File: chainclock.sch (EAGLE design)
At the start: 15 parts

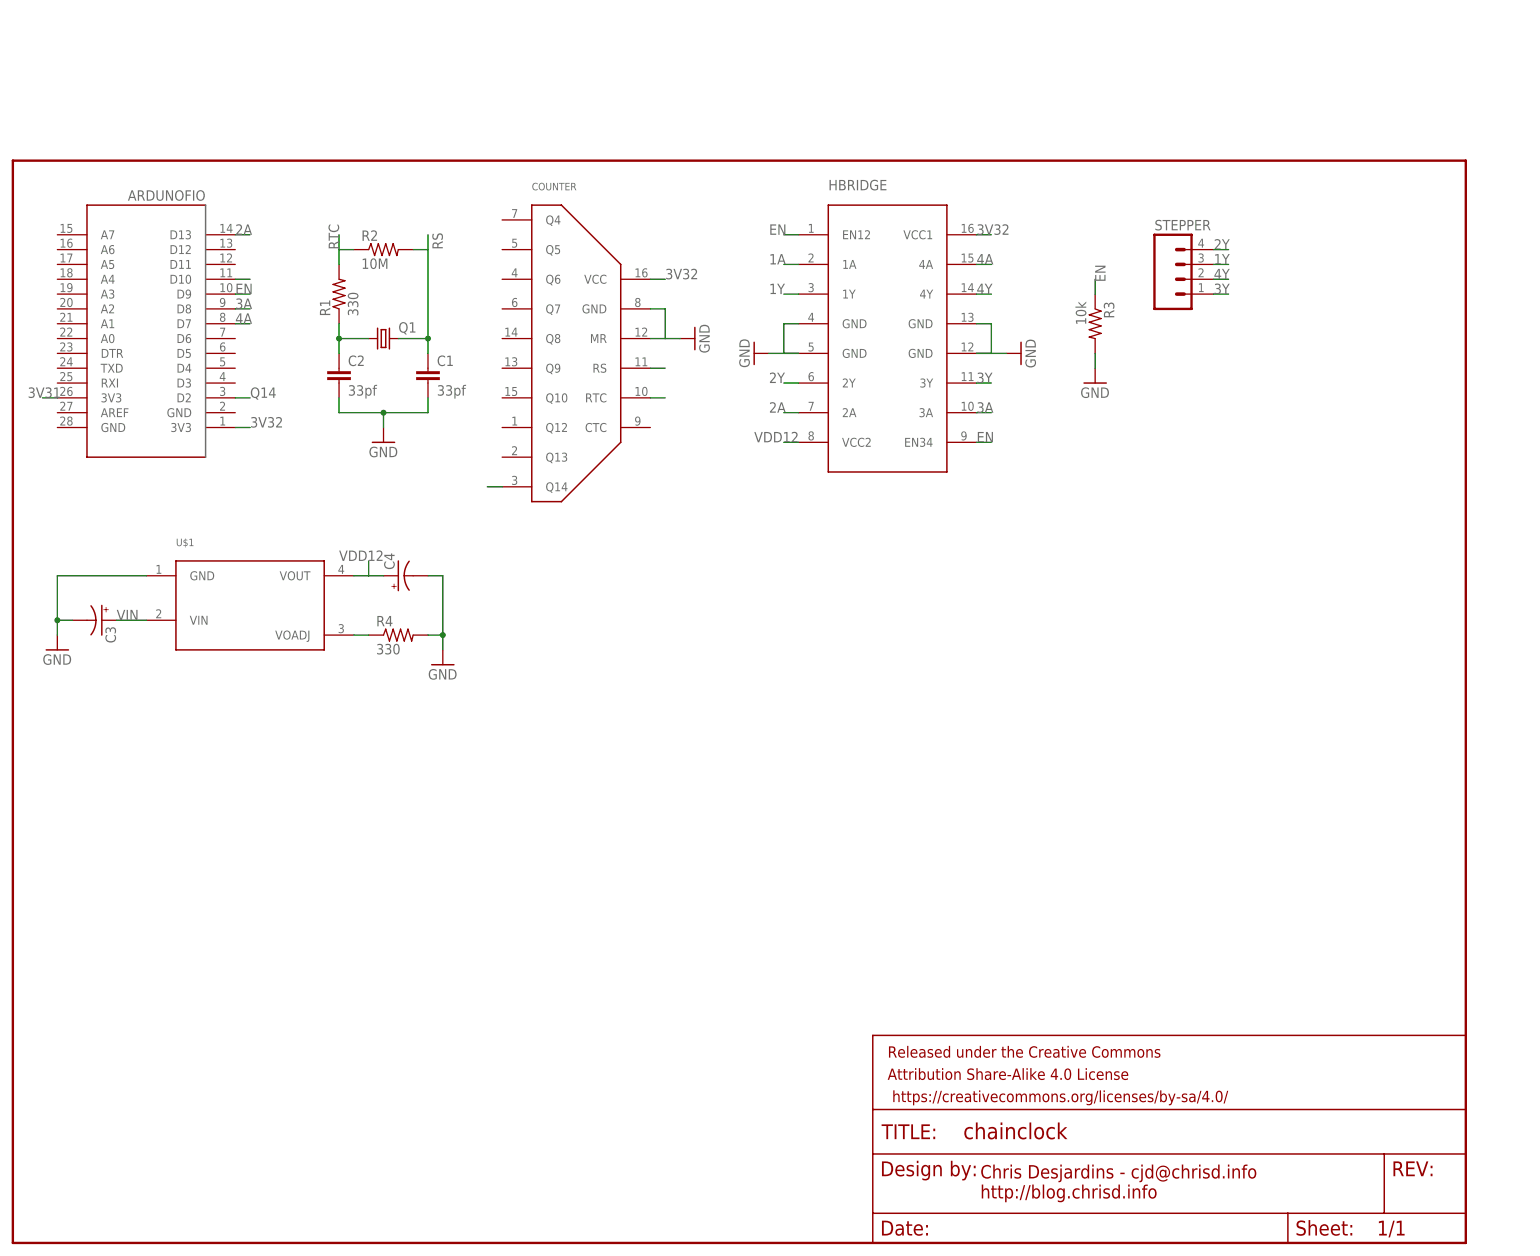
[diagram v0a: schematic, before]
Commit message: Move some stuff around
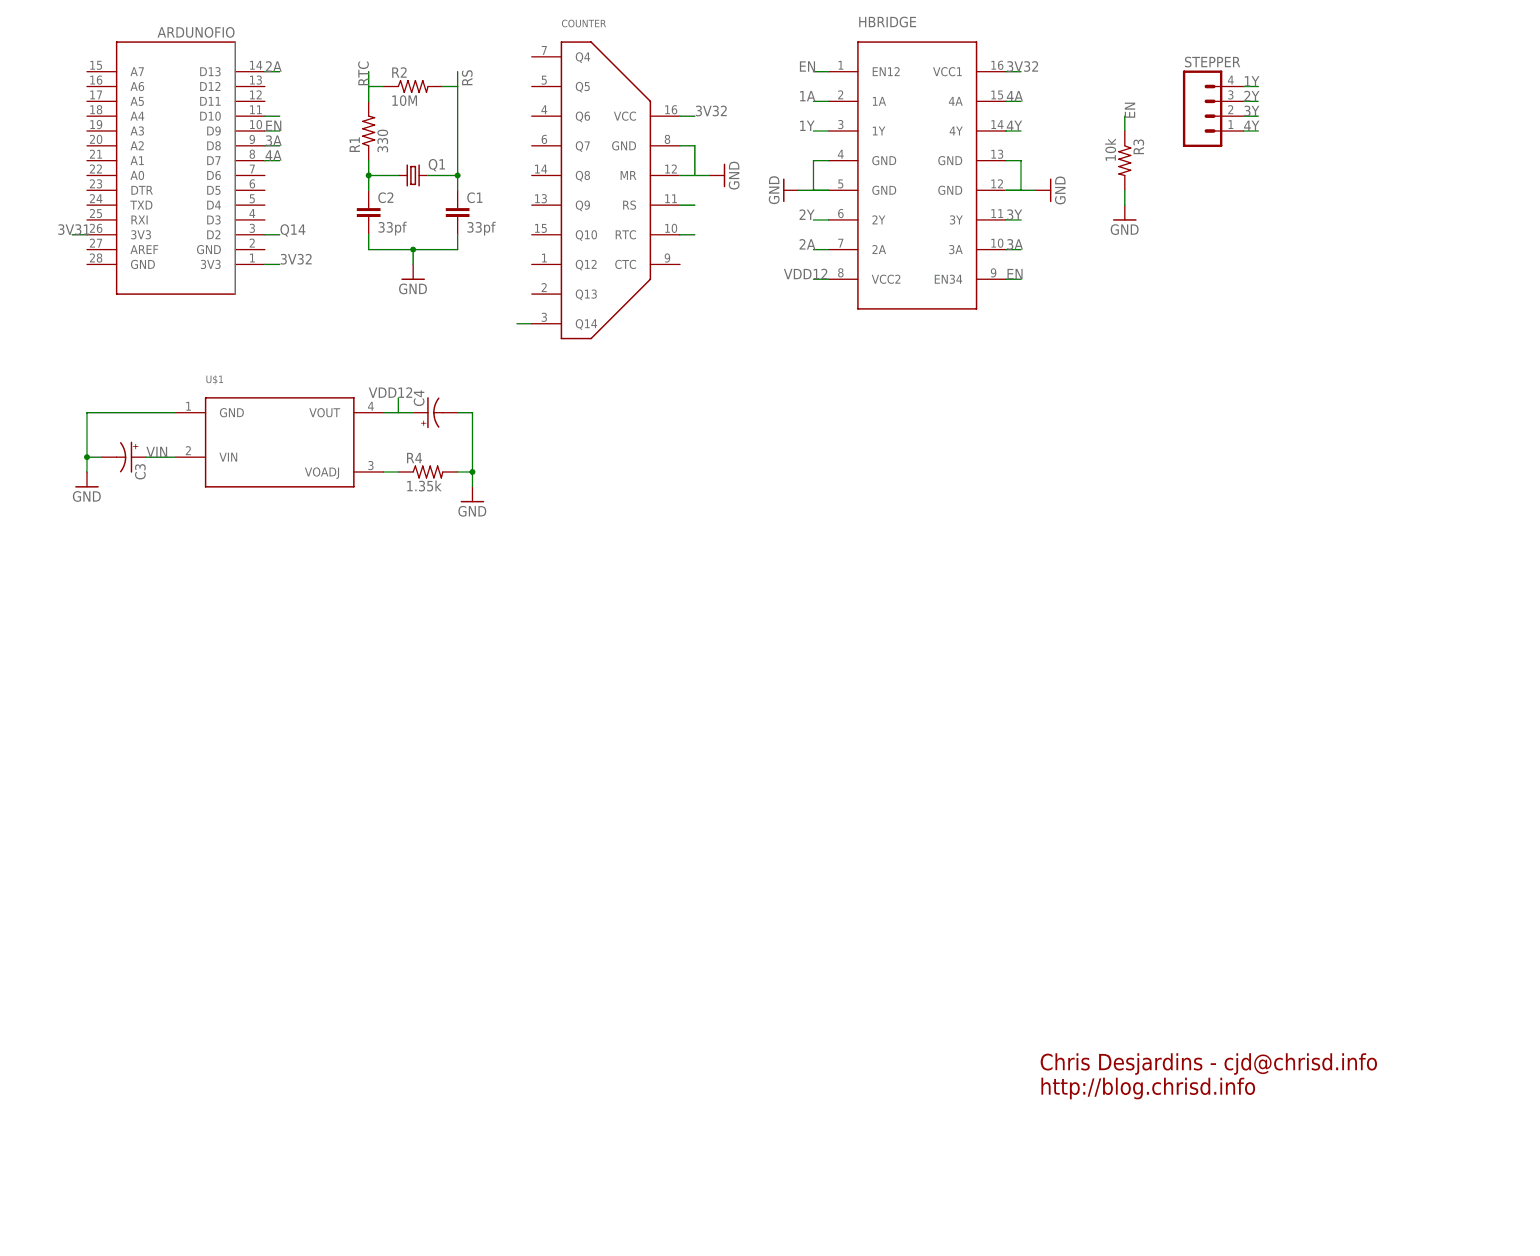
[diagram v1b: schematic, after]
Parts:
- removed FRAME1: FRAME-LETTER, SparkFun-Aesthetics:FRAME-LETTER
- R4: value 330 -> 1.35k
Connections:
- net 1Y: now also STEPPER.4; no longer STEPPER.3
- net 2Y: now also STEPPER.3; no longer STEPPER.4
- net 3Y: now also STEPPER.2; no longer STEPPER.1
- net 4Y: now also STEPPER.1; no longer STEPPER.2
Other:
- moved on the sheet: ARDUNOFIO, C1, C2, C3, C4, COUNTER, HBRIDGE, Q1, R1, R2, R3, R4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
